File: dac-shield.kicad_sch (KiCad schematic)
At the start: 44 parts, among them J1 Conn_01x02, J2 Conn_01x02, J3 Conn_01x02, J4 Conn_01x02, J5 Conn_01x02, J6 Conn_01x02, J7 Conn_01x02, J8 Conn_01x02

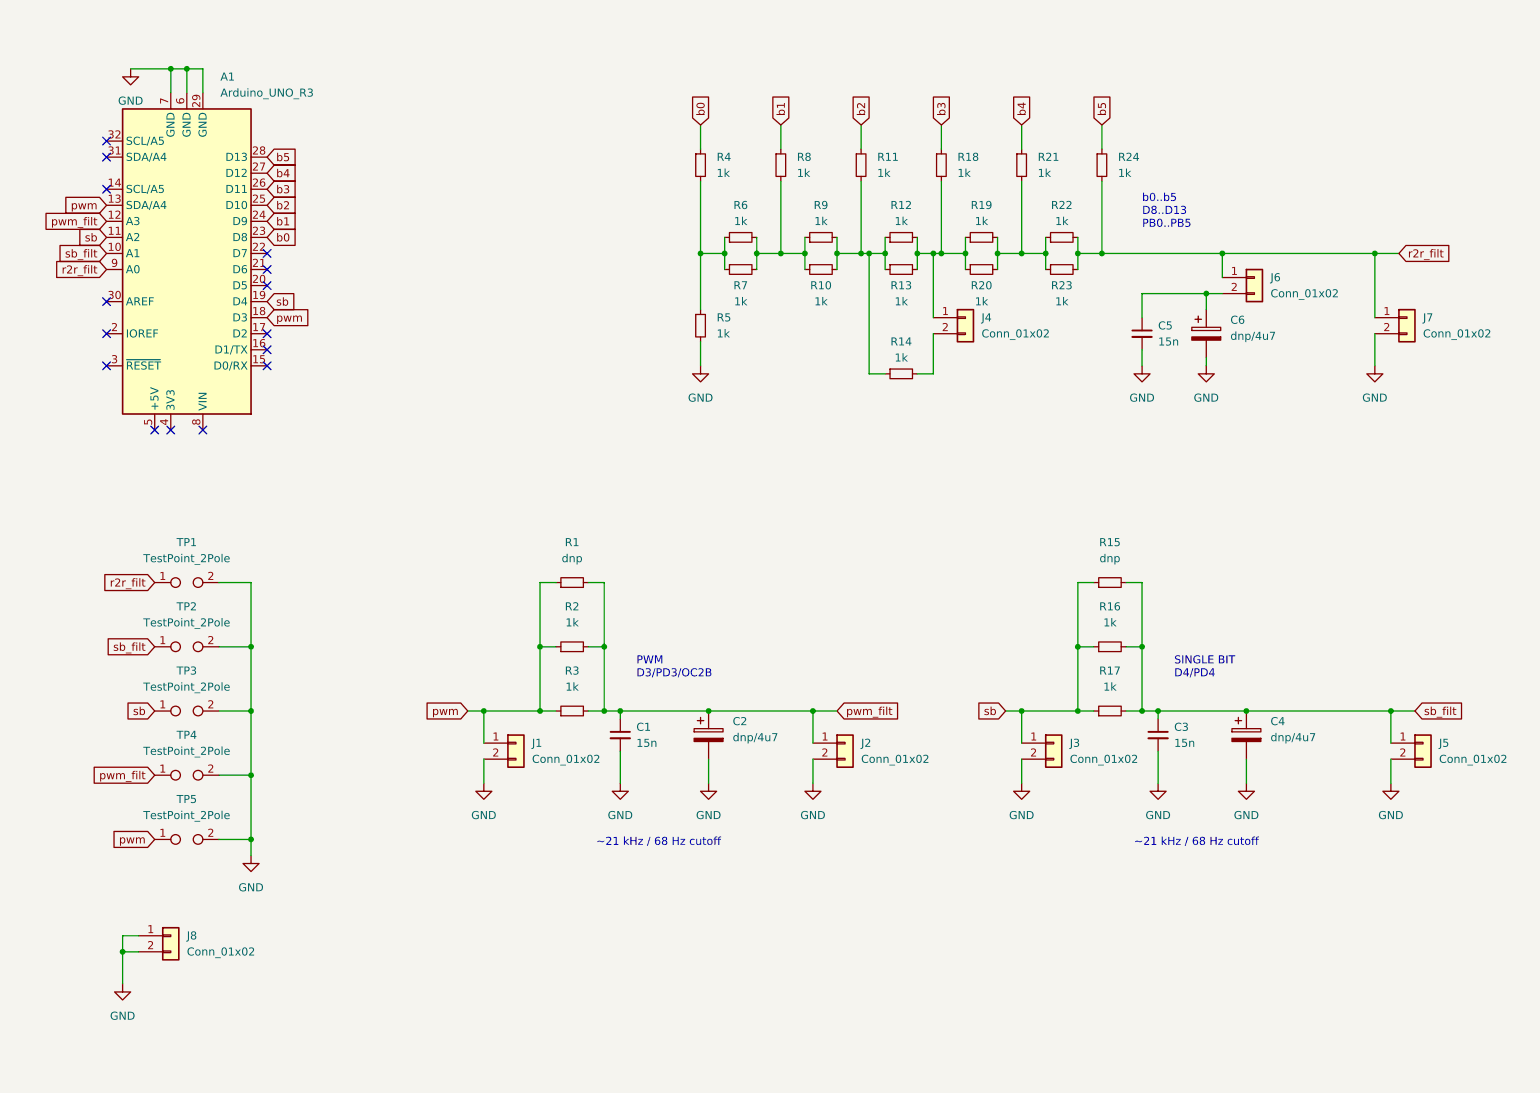
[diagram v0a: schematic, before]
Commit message: prettified things
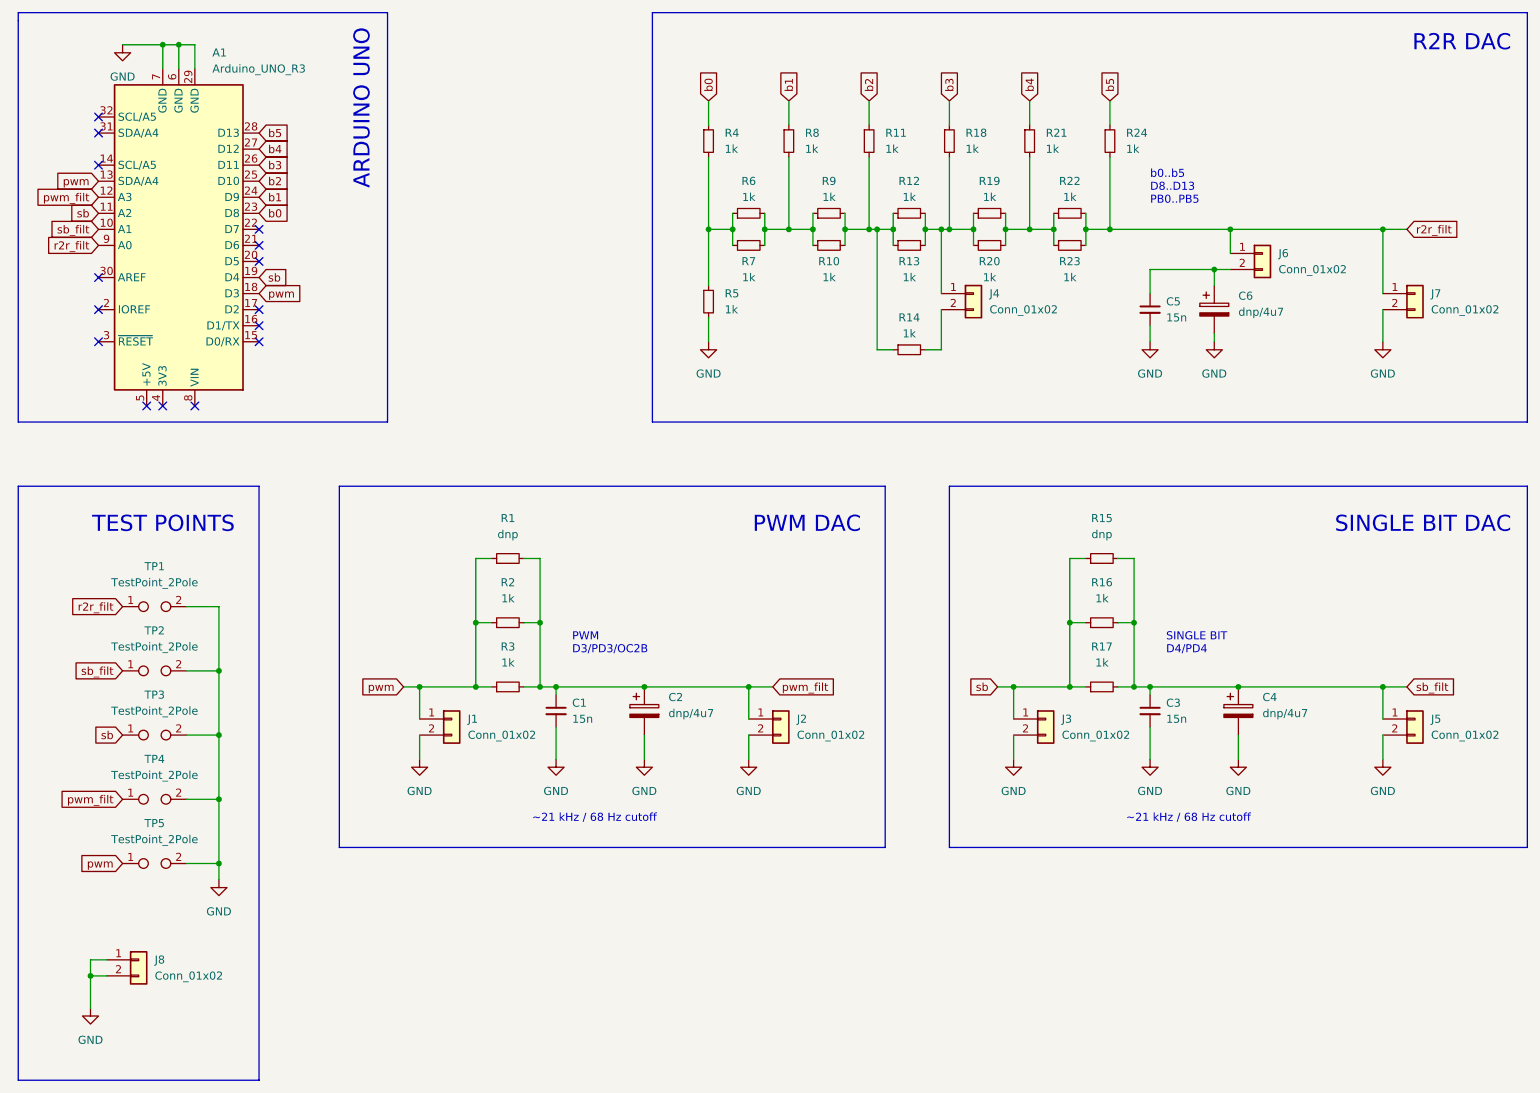
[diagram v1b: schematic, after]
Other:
- note added: "ARDUINO UNO"
- note added: "PWM DAC"
- note added: "R2R DAC"
- note added: "SINGLE BIT DAC"
- note added: "TEST POINTS"
- moved on the sheet: A1, C1, C2, C3, C4, C5, C6, J1, J2, J3, J4, J5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
